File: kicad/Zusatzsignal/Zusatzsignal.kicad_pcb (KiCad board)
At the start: 2 copper layers, 3.7 x 5.3 mm, 3 parts, among them J1 VCC, J2 Zs

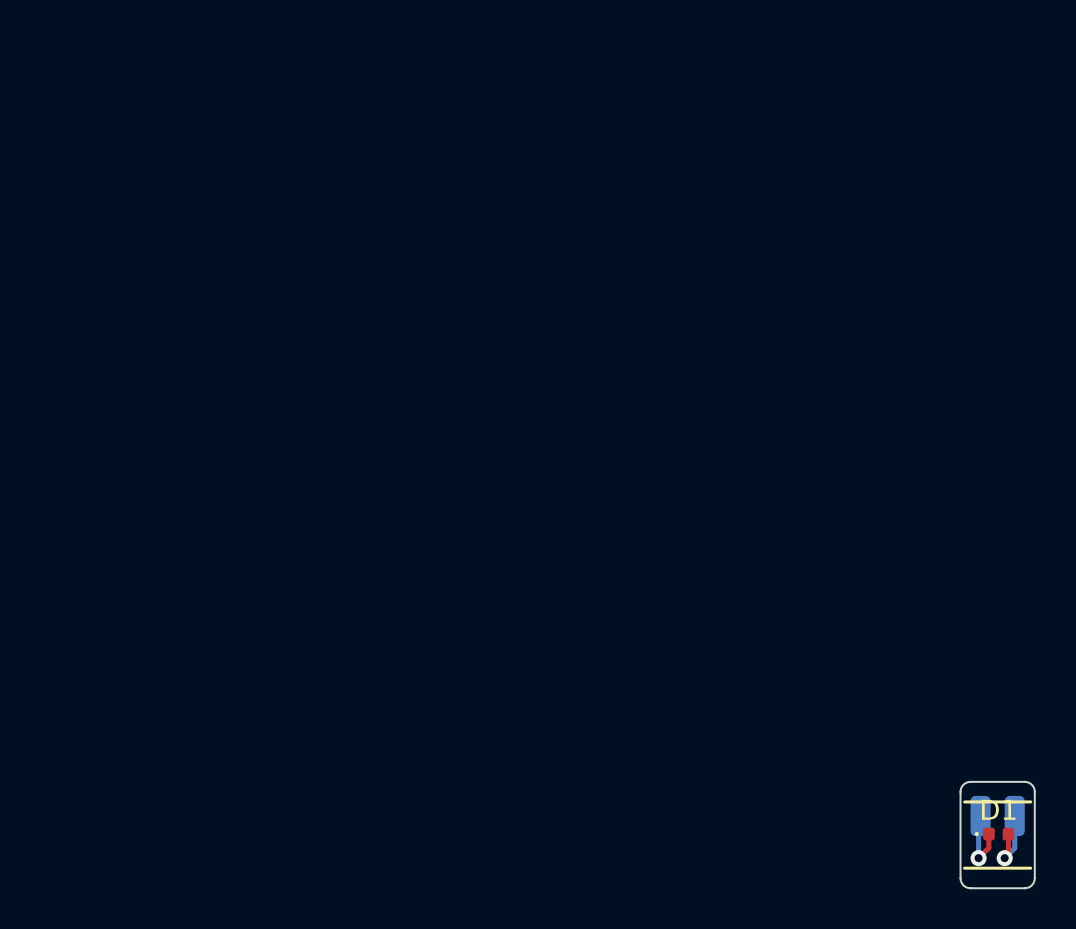
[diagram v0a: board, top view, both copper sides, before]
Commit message: Add CC-BY-SA 4.0 license
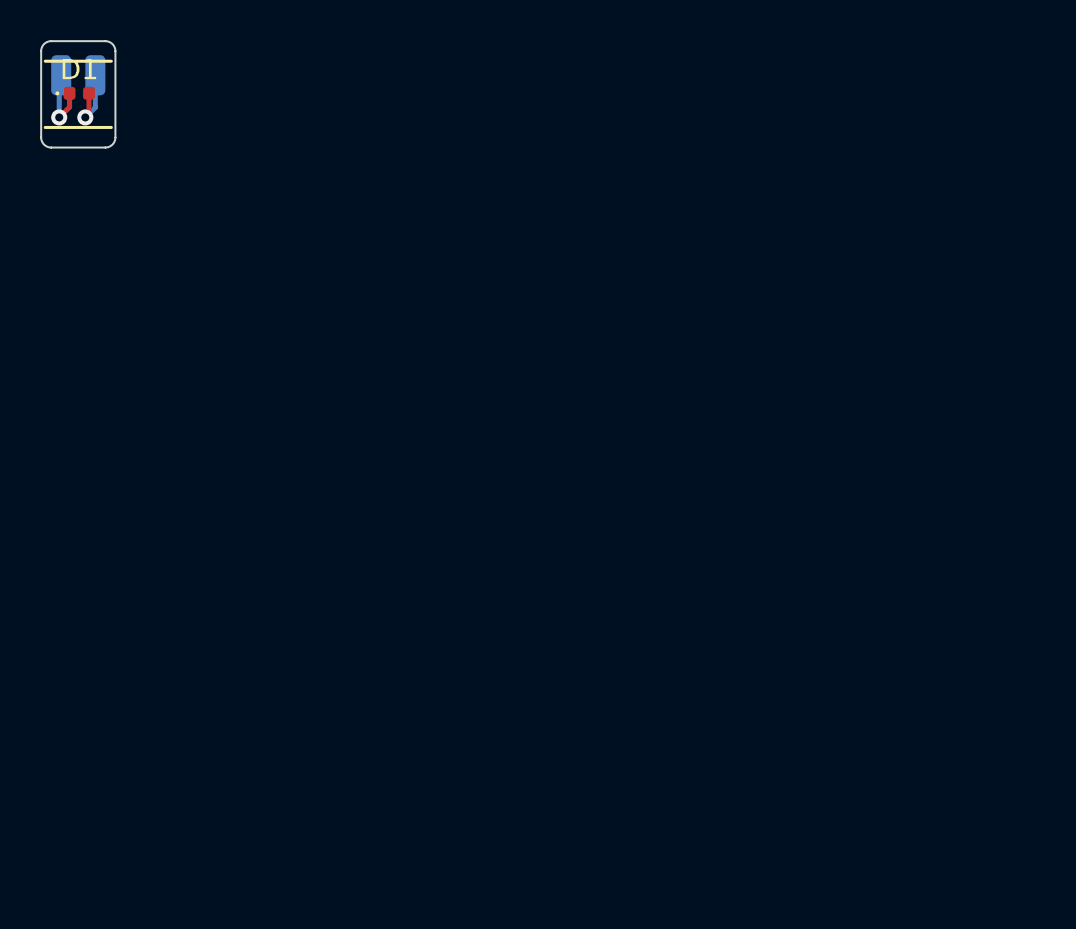
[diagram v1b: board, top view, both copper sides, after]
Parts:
- moved D1 58.8 mm to (98.4, 65.6)
- moved J2 58.8 mm to (97.5, 64.7)
- moved J1 58.8 mm to (99.2, 64.7)
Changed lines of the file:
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@@
     (thickness 0.8)
   )
-  (paper "A4")
+  (paper "A5")
   (title_block
-    (title "ZS")
+    (title "KS-Zusatzsignal")
+    (date "2023-12-17")
     (rev "v3")
-    (comment 4 "AISLER Project ID: DXIHIPTI")
   )
   (layers
@@
     )
     (pad_to_mask_clearance 0)
+    (aux_axis_origin 96.5 63)
     (pcbplotparams
       (layerselection 0x00010fc_ffffffff)
@@
   (net 2 "Net-(D1-Pad1)")
   (footprint "LED_SMD:LED_0402_1005Metric" (layer "F.Cu")
-    (at 144.2 102.5)
+    (at 98.4 65.6)
     (descr "LED SMD 0402 (1005 Metric), square (rectangular) end terminal, IPC_7351 nominal, (Body size source: http://www.tortai-tech.com/upload/download/2011102023233369053.pdf), generated with kicad-footprint-generator")
     (tags "LED")
@@
   )
   (footprint "Connector_Wire:SolderWirePad_1x01_SMD_1x2mm" (layer "B.Cu")
-    (at 143.3 101.6 180)
+    (at 97.5 64.7 180)
     (descr "Wire Pad, Square, SMD Pad,  5mm x 10mm,")
     (tags "MesurementPoint Square SMDPad 5mmx10mm ")
@@
   )
   (footprint "Connector_Wire:SolderWirePad_1x01_SMD_1x2mm" (layer "B.Cu")
-    (at 145 101.6 180)
+    (at 99.2 64.7 180)
     (descr "Wire Pad, Square, SMD Pad,  5mm x 10mm,")
     (tags "MesurementPoint Square SMDPad 5mmx10mm ")
@@
       (net 1 "Net-(D1-Pad2)") (pinfunction "Pin_1") (pintype "passive"))
   )
-  (gr_line (start 145.8 100.9) (end 142.5 100.9)
+  (gr_line (start 100 64) (end 96.7 64)
     (stroke (width 0.15) (type solid)) (layer "F.SilkS"))
-  (gr_line (start 145.8 104.2) (end 142.5 104.2)
+  (gr_line (start 100 67.3) (end 96.7 67.3)
     (stroke (width 0.15) (type solid)) (layer "F.SilkS"))
-  (gr_line (start 142.8 99.9) (end 145.5 99.9)
-    (stroke (width 0.1) (type solid)) (layer "Edge.Cuts"))
-  (gr_arc (start 142.3 100.4) (mid 142.446447 100.046447) (end 142.8 99.9)
-    (stroke (width 0.1) (type solid)) (layer "Edge.Cuts"))
-  (gr_line (start 146 100.4) (end 146 104.7)
-    (stroke (width 0.1) (type solid)) (layer "Edge.Cuts"))
-  (gr_line (start 142.3 104.7) (end 142.3 100.4)
-    (stroke (width 0.1) (type solid)) (layer "Edge.Cuts"))
-  (gr_arc (start 145.5 99.9) (mid 145.853553 100.046447) (end 146 100.4)
-    (stroke (width 0.1) (type solid)) (layer "Edge.Cuts"))
-  (gr_arc (start 146 104.7) (mid 145.853553 105.053553) (end 145.5 105.2)
-    (stroke (width 0.1) (type solid)) (layer "Edge.Cuts"))
-  (gr_line (start 145.5 105.2) (end 142.8 105.2)
-    (stroke (width 0.1) (type solid)) (layer "Edge.Cuts"))
-  (gr_arc (start 142.8 105.2) (mid 142.446447 105.053553) (end 142.3 104.7)
-    (stroke (width 0.1) (type solid)) (layer "Edge.Cuts"))
-  (gr_text "+" (at 145 103.1) (layer "B.SilkS")
+  (gr_line (start 97 63) (end 99.7 63)
+    (stroke (width 0.1) (type solid)) (layer "Edge.Cuts"))
+  (gr_arc (start 96.5 63.5) (mid 96.646447 63.146447) (end 97 63)
+    (stroke (width 0.1) (type solid)) (layer "Edge.Cuts"))
+  (gr_line (start 100.2 63.5) (end 100.2 67.8)
+    (stroke (width 0.1) (type solid)) (layer "Edge.Cuts"))
+  (gr_line (start 96.5 67.8) (end 96.5 63.5)
+    (stroke (width 0.1) (type solid)) (layer "Edge.Cuts"))
+  (gr_arc (start 99.7 63) (mid 100.053553 63.146447) (end 100.2 63.5)
+    (stroke (width 0.1) (type solid)) (layer "Edge.Cuts"))
+  (gr_arc (start 100.2 67.8) (mid 100.053553 68.153553) (end 99.7 68.3)
+    (stroke (width 0.1) (type solid)) (layer "Edge.Cuts"))
+  (gr_line (start 99.7 68.3) (end 97 68.3)
+    (stroke (width 0.1) (type solid)) (layer "Edge.Cuts"))
+  (gr_arc (start 97 68.3) (mid 96.646447 68.153553) (end 96.5 67.8)
+    (stroke (width 0.1) (type solid)) (layer "Edge.Cuts"))
+  (gr_text "+" (at 99.2 66.2) (layer "B.SilkS")
     (effects (font (size 1 1) (thickness 0.15)) (justify mirror))
   )
-  (gr_text "ZSv3" (at 144.1 104.5) (layer "B.SilkS")
+  (gr_text "ZSv3" (at 98.3 67.6) (layer "B.SilkS")
     (effects (font (size 0.8 0.8) (thickness 0.15)) (justify mirror))
   )
-  (segment (start 144.685 102.5) (end 144.685 103.515) (width 0.25) (layer "F.Cu") (net 1))
-  (segment (start 144.685 103.515) (end 144.5 103.7) (width 0.25) (layer "F.Cu") (net 1))
-  (via (at 144.5 103.7) (size 0.8) (drill 0.4) (layers "F.Cu" "B.Cu") (net 1))
-  (segment (start 145 101.6) (end 145 103.2) (width 0.25) (layer "B.Cu") (net 1))
-  (segment (start 145 103.2) (end 144.5 103.7) (width 0.25) (layer "B.Cu") (net 1))
-  (segment (start 143.715 103.185) (end 143.2 103.7) (width 0.25) (layer "F.Cu") (net 2))
-  (segment (start 143.715 102.5) (end 143.715 103.185) (width 0.25) (layer "F.Cu") (net 2))
-  (via (at 143.2 103.7) (size 0.8) (drill 0.4) (layers "F.Cu" "B.Cu") (net 2))
-  (segment (start 143.2 103.7) (end 143.2 101.7) (width 0.25) (layer "B.Cu") (net 2))
-  (segment (start 143.2 101.7) (end 143.3 101.6) (width 0.25) (layer "B.Cu") (net 2))
-  (segment (start 143.25 101.65) (end 143.3 101.6) (width 0.25) (layer "B.Cu") (net 2))
-  (arc (start 143.25 101.65) (mid 143.212994 101.705382) (end 143.2 101.77071) (width 0.25) (layer "B.Cu") (net 2))
+  (segment (start 98.885 65.6) (end 98.885 66.615) (width 0.25) (layer "F.Cu") (net 1))
+  (segment (start 98.885 66.615) (end 98.7 66.8) (width 0.25) (layer "F.Cu") (net 1))
+  (via (at 98.7 66.8) (size 0.8) (drill 0.4) (layers "F.Cu" "B.Cu") (net 1))
+  (segment (start 99.2 64.7) (end 99.2 66.3) (width 0.25) (layer "B.Cu") (net 1))
+  (segment (start 99.2 66.3) (end 98.7 66.8) (width 0.25) (layer "B.Cu") (net 1))
+  (segment (start 97.915 66.285) (end 97.4 66.8) (width 0.25) (layer "F.Cu") (net 2))
+  (segment (start 97.915 65.6) (end 97.915 66.285) (width 0.25) (layer "F.Cu") (net 2))
+  (via (at 97.4 66.8) (size 0.8) (drill 0.4) (layers "F.Cu" "B.Cu") (net 2))
+  (segment (start 97.4 66.8) (end 97.4 64.8) (width 0.25) (layer "B.Cu") (net 2))
+  (segment (start 97.4 64.8) (end 97.5 64.7) (width 0.25) (layer "B.Cu") (net 2))
+  (segment (start 97.45 64.75) (end 97.5 64.7) (width 0.25) (layer "B.Cu") (net 2))
+  (arc (start 97.45 64.75) (mid 97.412994 64.805382) (end 97.4 64.87071) (width 0.25) (layer "B.Cu") (net 2))
 )
